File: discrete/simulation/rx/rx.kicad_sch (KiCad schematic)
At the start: 21 parts, among them Q1 2N5551, Q2 2N5401, Q3 2N5401

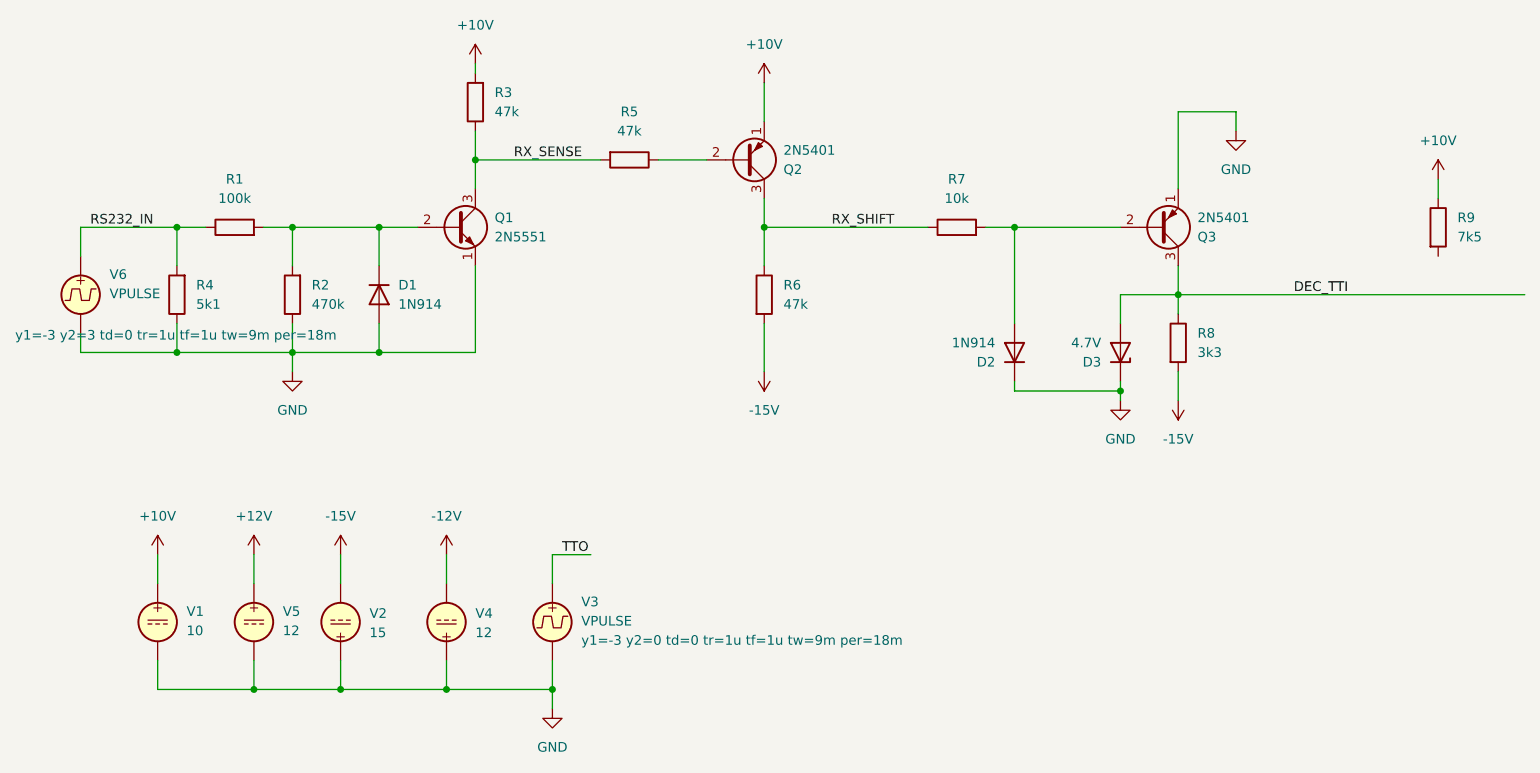
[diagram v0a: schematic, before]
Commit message: Final Rx modeling
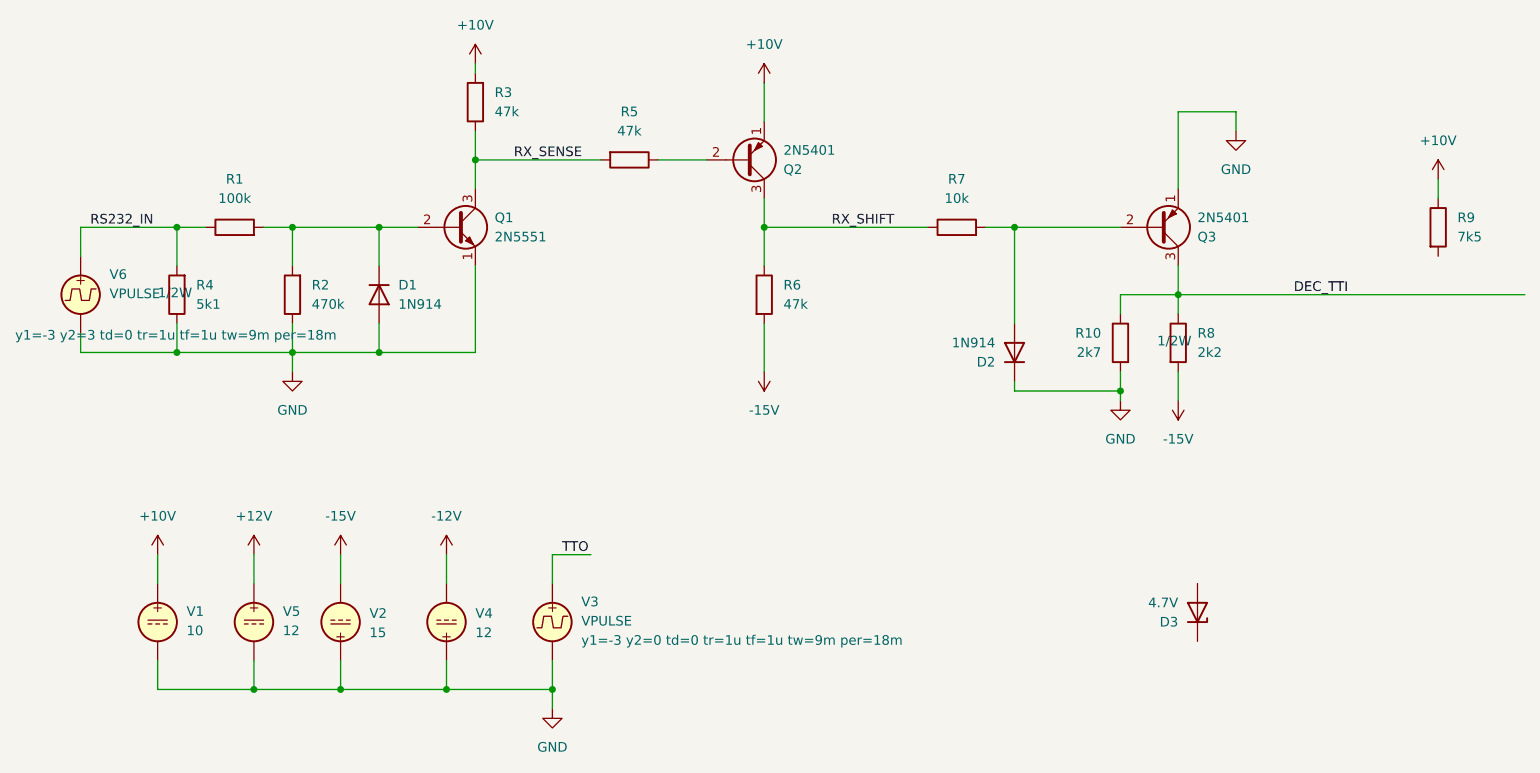
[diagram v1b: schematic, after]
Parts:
- added R10: 2k7, symbol Device:R
- R8: value 3k3 -> 2k2
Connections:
- net DEC_TTI: now also R10.1; no longer D3.2 (A)
- net GND: now also R10.2; no longer D3.1 (K)
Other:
- note added: "1/2W"
- moved on the sheet: D3
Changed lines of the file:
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@@
 	(generator_version "9.0")
 	(paper "A4")
+	(text "1/2W"
+		(exclude_from_sim no)
+		(at 37.846 71.12 0)
+		(effects
+			(font
+				(size 1.27 1.27)
+			)
+		)
+	)
+	(text "1/2W"
+		(exclude_from_sim no)
+		(at 169.672 77.47 0)
+		(effects
+			(font
+				(size 1.27 1.27)
+			)
+		)
+	)
 	(junction
 		(at 73.66 123.19)
@@
 	(wire
 		(pts
-			(xy 162.56 74.93) (xy 162.56 71.12)
+			(xy 170.18 71.12) (xy 215.9 71.12)
+		)
+		(stroke
+			(width 0)
+			(type default)
+		)
+	)
+	(wire
+		(pts
+			(xy 162.56 73.66) (xy 162.56 71.12)
 		)
 		(stroke
@@
 	(wire
 		(pts
-			(xy 162.56 82.55) (xy 162.56 83.82)
-		)
-		(stroke
-			(width 0)
-			(type default)
-		)
-	)
-	(wire
-		(pts
-			(xy 170.18 71.12) (xy 215.9 71.12)
+			(xy 162.56 81.28) (xy 162.56 83.82)
 		)
 		(stroke
@@
 			)
 		)
-		(property "Value" "3k3"
+		(property "Value" "2k2"
 			(at 172.72 78.7399 0)
 			(effects
@@
 	(symbol
 		(lib_id "Device:D_Zener")
-		(at 162.56 78.74 270)
+		(at 172.72 113.03 270)
 		(mirror x)
 		(unit 1)
@@
 		(dnp no)
 		(property "Reference" "D3"
-			(at 160.02 80.0101 90)
+			(at 170.18 114.3001 90)
 			(effects
 				(font
@@
 		)
 		(property "Value" "4.7V"
-			(at 160.02 77.4701 90)
+			(at 170.18 111.7601 90)
 			(effects
 				(font
@@
 		)
 		(property "Footprint" ""
-			(at 162.56 78.74 0)
+			(at 172.72 113.03 0)
 			(effects
 				(font
@@
 		)
 		(property "Datasheet" "~"
-			(at 162.56 78.74 0)
+			(at 172.72 113.03 0)
 			(effects
 				(font
@@
 		)
 		(property "Description" "Zener diode"
-			(at 162.56 78.74 0)
+			(at 172.72 113.03 0)
 			(effects
 				(font
@@
 		)
 		(property "Sim.Library" "/home/sfinneran/work/ACMS/PDP-8-Serial/discrete/simulation/models/zener_4v7.lib"
-			(at 162.56 78.74 0)
+			(at 172.72 113.03 0)
 			(effects
 				(font
@@
 		)
 		(property "Sim.Name" "D4V7"
-			(at 162.56 78.74 0)
+			(at 172.72 113.03 0)
 			(effects
 				(font
@@
 		)
 		(property "Sim.Device" "D"
-			(at 162.56 78.74 0)
+			(at 172.72 113.03 0)
 			(effects
 				(font
@@
 		)
 		(property "Sim.Pins" "1=K 2=A"
-			(at 162.56 78.74 0)
+			(at 172.72 113.03 0)
 			(effects
 				(font
@@
 					(unit 1)
 				)
+			)
+		)
+	)
+	(symbol
+		(lib_id "Device:R")
+		(at 162.56 77.47 0)
+		(mirror y)
+		(unit 1)
+		(exclude_from_sim no)
+		(in_bom yes)
+		(on_board yes)
+		(dnp no)
+		(property "Reference" "R10"
+			(at 160.02 76.1999 0)
+			(effects
+				(font
+					(size 1.27 1.27)
+				)
+				(justify left)
+			)
+		)
+		(property "Value" "2k7"
+			(at 160.02 78.7399 0)
+			(effects
+				(font
+					(size 1.27 1.27)
+				)
+				(justify left)
+			)
+		)
+		(property "Footprint" ""
+			(at 164.338 77.47 90)
+			(effects
+				(font
+					(size 1.27 1.27)
+				)
+				(hide yes)
+			)
+		)
+		(property "Datasheet" "~"
+			(at 162.56 77.47 0)
+			(effects
+				(font
+					(size 1.27 1.27)
+				)
+				(hide yes)
+			)
+		)
+		(property "Description" "Resistor"
+			(at 162.56 77.47 0)
+			(effects
+				(font
+					(size 1.27 1.27)
+				)
+				(hide yes)
+			)
+		)
+		(pin "1"
+		)
+		(pin "2"
+		)
+		(instances
+			(project "rx"
+				(path "/f7e369c0-c7d8-4213-ba85-708f7769f576"
+					(reference "R10")
+					(unit 1)
+				)
